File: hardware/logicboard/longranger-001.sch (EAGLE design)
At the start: 25 parts, among them IC1 74ALS05N, IC2 LTC485N, IC3 LTC485N

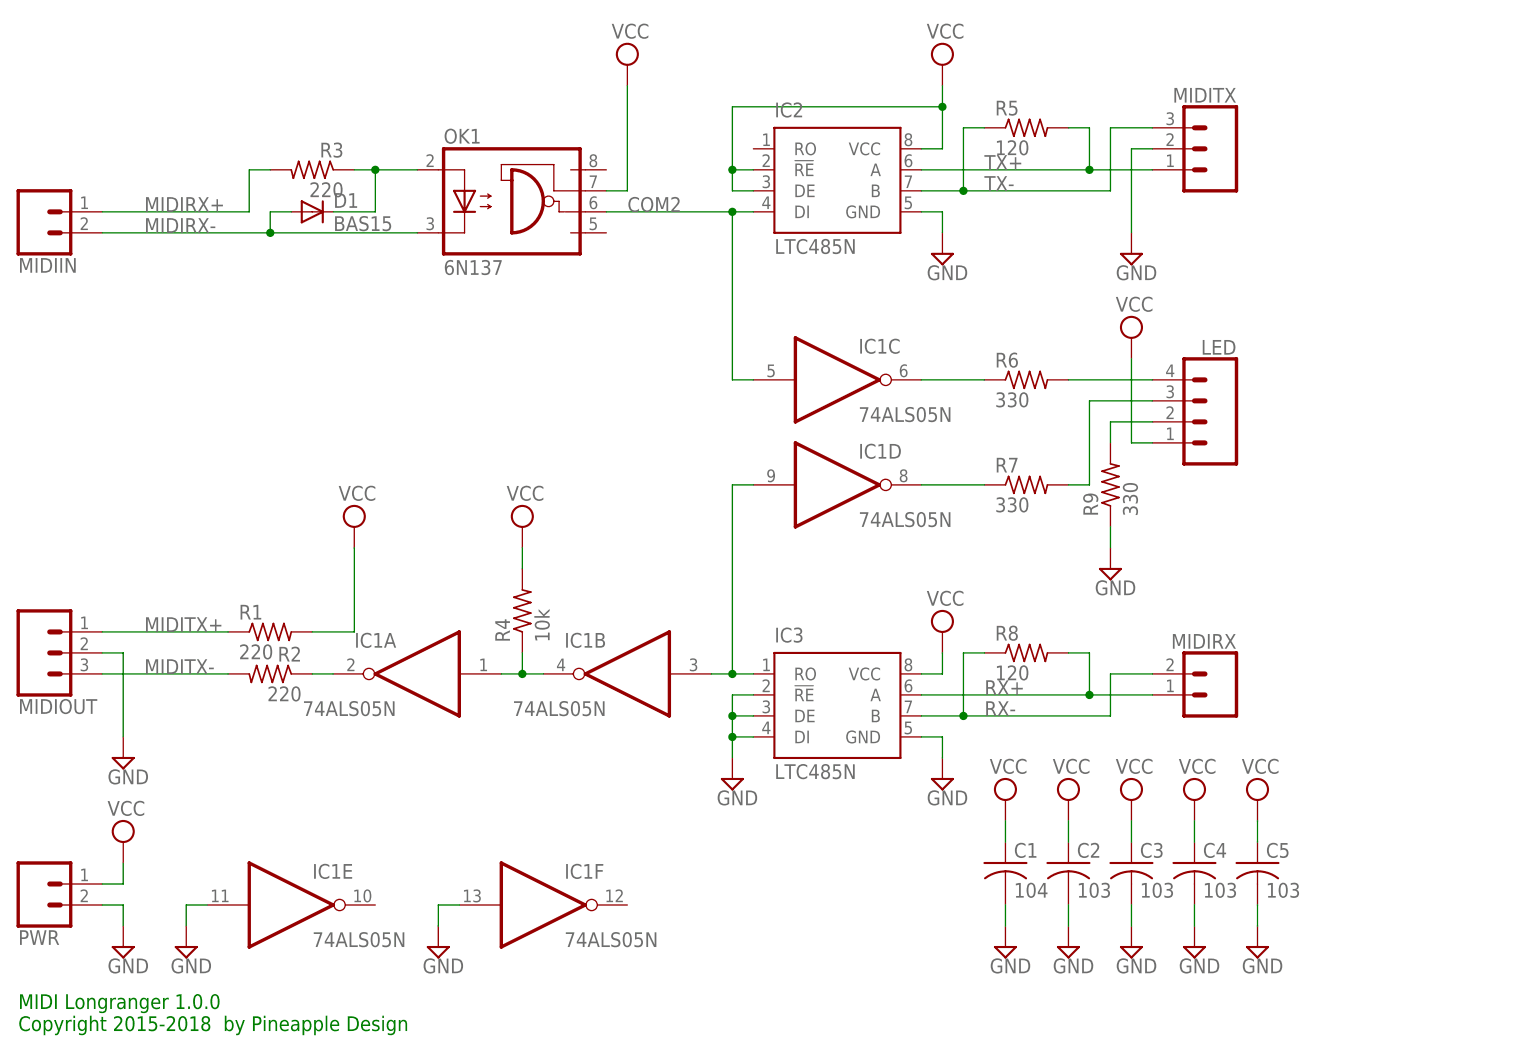
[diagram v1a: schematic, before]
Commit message: Renew.
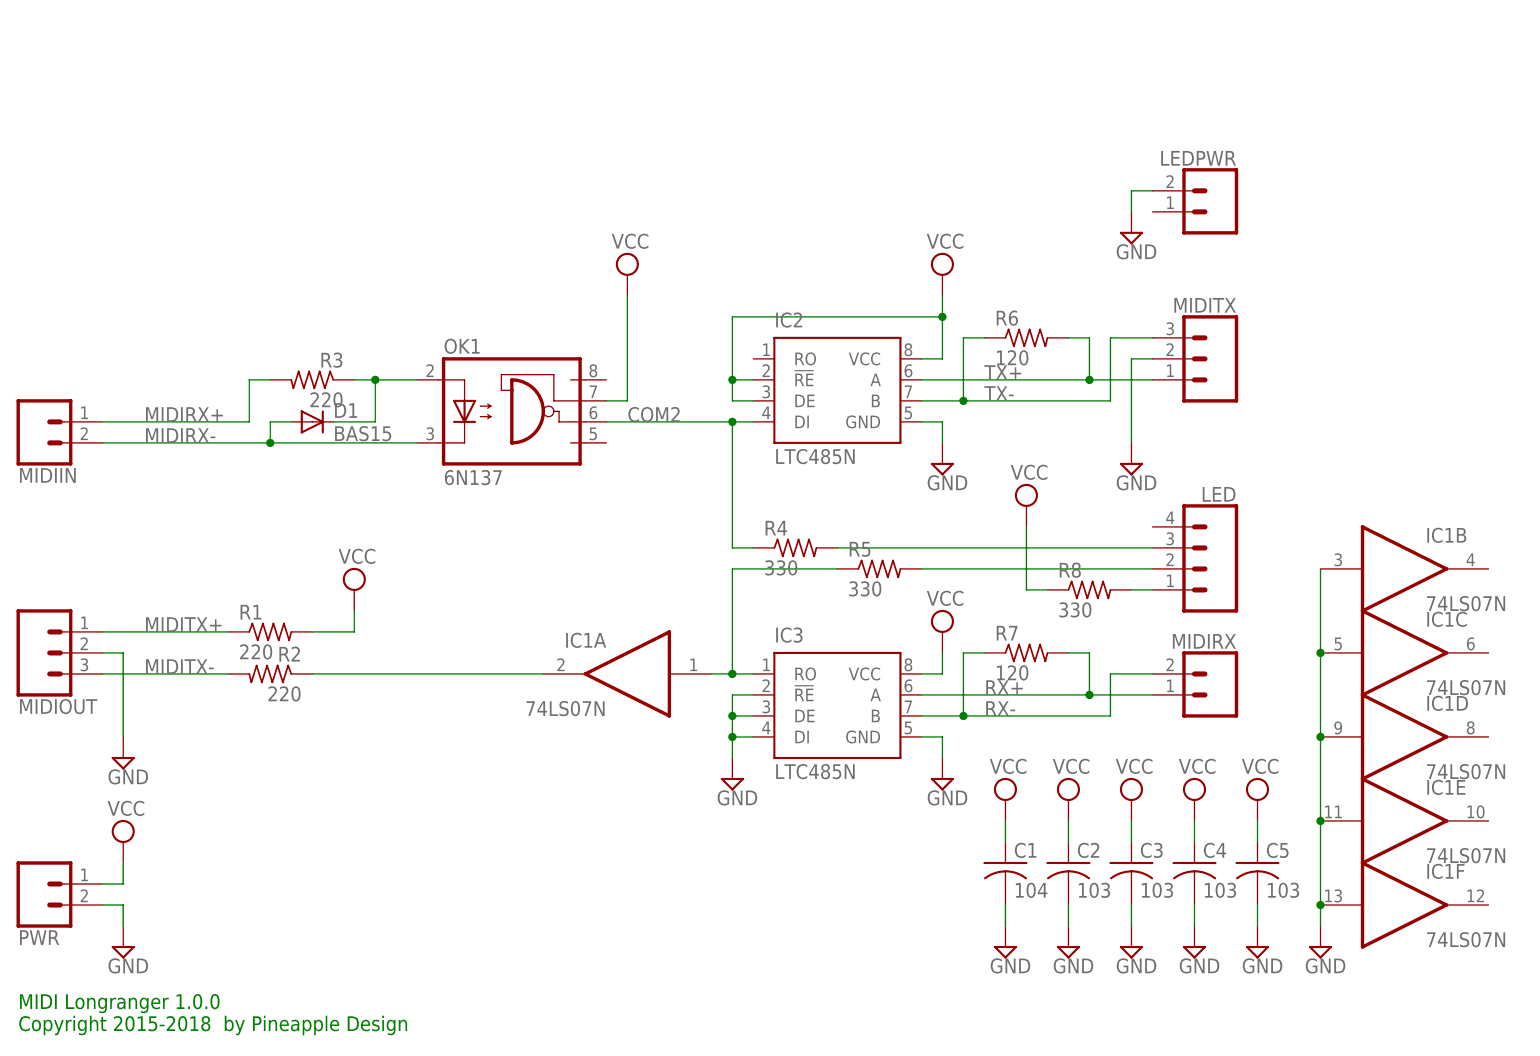
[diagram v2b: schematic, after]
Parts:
- removed R9: 330, resistor:R-US_0204/5
- added LEDPWR: (no value), SparkFun-Connectors:CONN_02JST-PTH-2
- IC1: value 74ALS05N -> 74LS07N; device 74xx-eu:74ALS05N -> 74xx-us:74LS07N
- R4: value 10k -> 330
- R5, R8: value 120 -> 330
- R6, R7: value 330 -> 120
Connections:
- removed net N$10: LED.2, R9.2
- removed net N$6: IC1C.O, R6.1
- removed net N$7: IC1D.O, R7.1
- removed net N$8: LED.4, R6.2
- removed net N$9: LED.3, R7.2
- new net N$4: LED.2, R5.2
- new net N$5: LED.3, R4.2
- net COM2: now also R4.1; no longer IC1C.I
- net GND: now also IC1B.I, IC1C.I, IC1D.I, LEDPWR.2; no longer R9.1
- net N$1: now also IC1A.I, R5.1; no longer IC1B.I, IC1D.I
- net N$3: now also LED.1, R8.2; no longer IC1A.I, IC1B.O, R4.1
- net RX+: now also R7.2; no longer R8.2
- net RX-: now also R7.1; no longer R8.1
- net TX+: now also R6.2; no longer R5.2
- net TX-: now also R6.1; no longer R5.1
- net VCC: now also R8.1; no longer LED.1, R4.2
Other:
- moved on the sheet: D1, IC2, LED, MIDIIN, MIDITX, OK1, R3, R4, R5, R6, R7, R8
